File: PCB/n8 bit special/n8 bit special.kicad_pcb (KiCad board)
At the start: 2 copper layers, 99.9 x 99.6 mm, 40 parts, among them J1 USB_B_Micro, J2 PORT0, J3 PORT2, J4 PORT1, J5 PORT3, J6 Conn_02x08_Odd_Even, SW1 SW_Push_Dual, U1 W65C02SxP, U2 CY62256-70PC, U3 CY62256-70PC, U4 28C256, U5 74LS21, U6 22V10C, U7 DS1813, X1 4Mhz

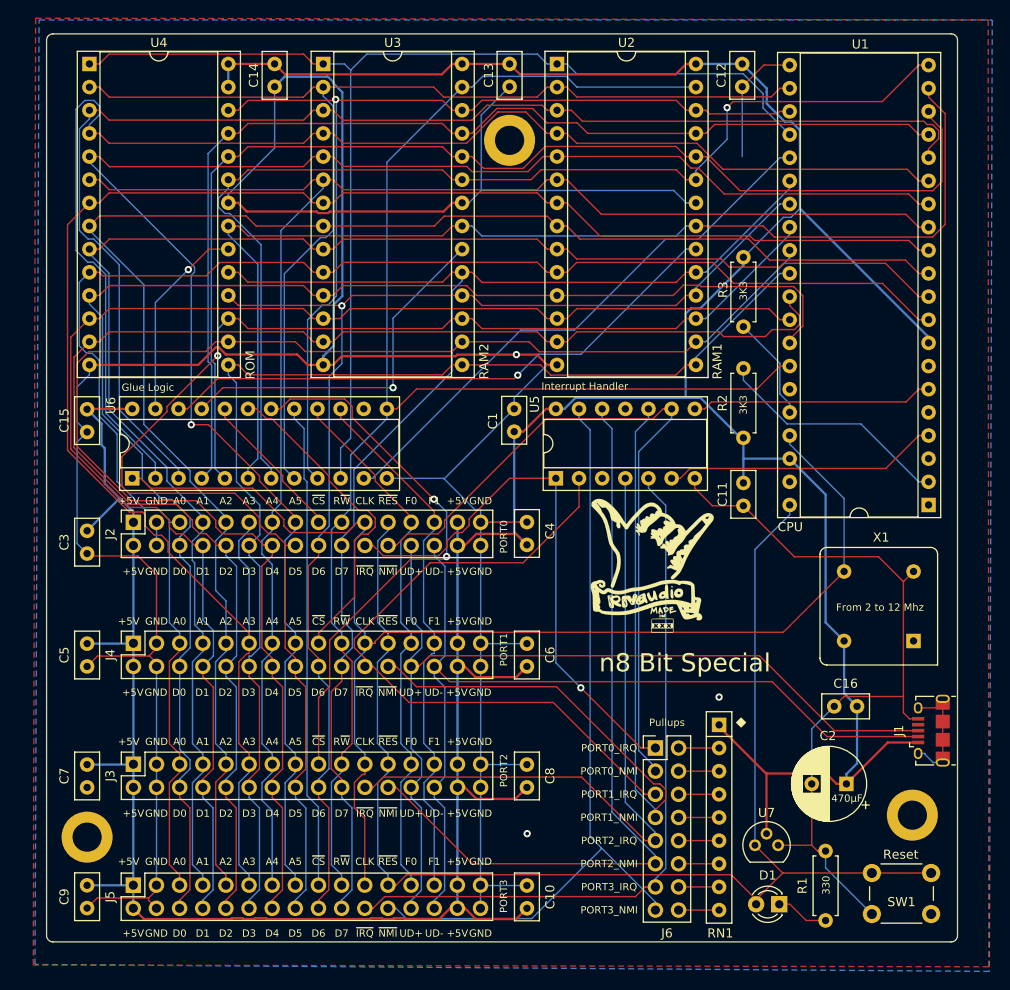
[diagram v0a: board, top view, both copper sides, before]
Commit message: v2 done
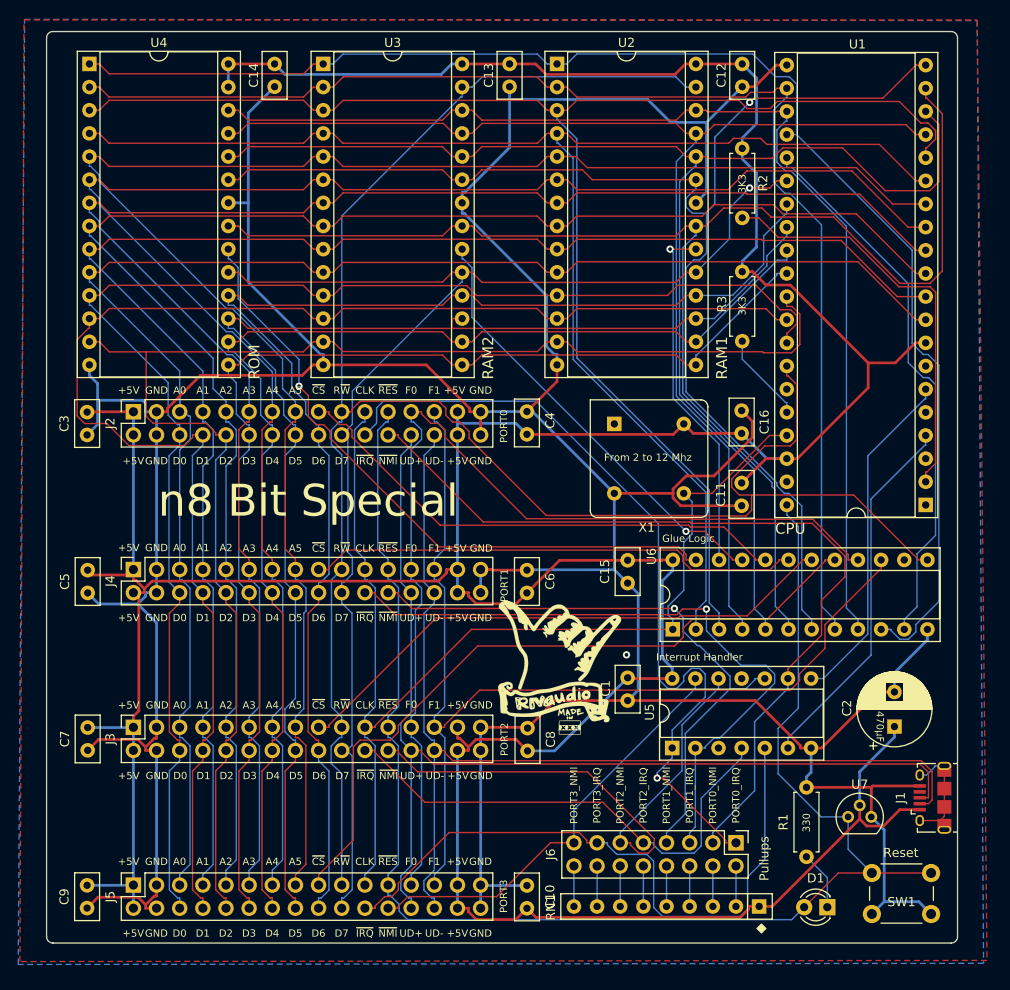
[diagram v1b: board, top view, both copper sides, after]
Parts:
- removed REF1, REF2, REF3: MountingHole_3.2mm_M3_DIN965_Pad, MountingHole:MountingHole_3.2mm_M3_DIN965_Pad
- moved C15 61.6 mm to (150.7, 100.4)
- moved U6 61.6 mm to (155.7, 105.5)
- moved X1 40.6 mm to (149.3, 82.9), turned to 270 degrees
- moved C1 34.3 mm to (150.7, 113.3), turned to 90 degrees
- moved C16 34.0 mm to (163.3, 81.5), turned to 270 degrees
- moved U5 32.2 mm to (155.6, 118.5)
- moved RN1 20.4 mm to (165.2, 135.9), turned to 180 degrees
- moved R2 16.5 mm to (163.3, 60.3), turned to 90 degrees
- moved G*** 15.1 mm to (143.2, 109.0)
- moved J6 13.6 mm to (162.6, 128.9), turned to 270 degrees
- moved C3 13.0 mm to (91.4, 84.1)
- moved C4 12.1 mm to (139.7, 84.1)
- moved J2 12.1 mm to (96.5, 81.6)
- moved U7 10.7 mm to (174.9, 126.0)
- moved C2 8.20 mm to (180.0, 116.1), turned to 90 degrees
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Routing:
- net FUTURE1: track 59.5 -> 114.5 mm
- net FUTURE0: track 59.3 -> 111.9 mm
- net R~W: track 169.1 -> 219.8 mm
- net ~ROM_CS: track 22.1 -> 71.9 mm
- net ~PORT0_CS: track 16.7 -> 56.4 mm
- net PORT3_NMI_PULLUP: track 85.6 -> 47.0 mm
- net PORT0_IRQ_PULLUP: track 60.8 -> 89.8 mm
- net /A10: track 126.7 -> 155.6 mm
- net /D4: track 163.7 -> 135.6 mm
- net /A14: track 128.6 -> 154.9 mm
- net ~PORT3_CS: track 53.4 -> 79.2 mm
- net ~RAM1_CS: track 64.0 -> 39.2 mm
- net /A11: track 122.4 -> 147.3 mm
- net PORT2_NMI_PULLUP: track 85.1 -> 61.4 mm
- net GND: track 453.3 -> 477.0 mm, vias 3 -> 1
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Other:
- board size 99.9 x 99.6 mm -> 99.9 x 100 mm
- net class Power: trace_width 0.25 -> 0.3
